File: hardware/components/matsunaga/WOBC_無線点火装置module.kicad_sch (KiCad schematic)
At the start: 24 parts, among them Q4 NPN, Q5 BS250, Q6 BS170, SW2 SW_DPDT_x2

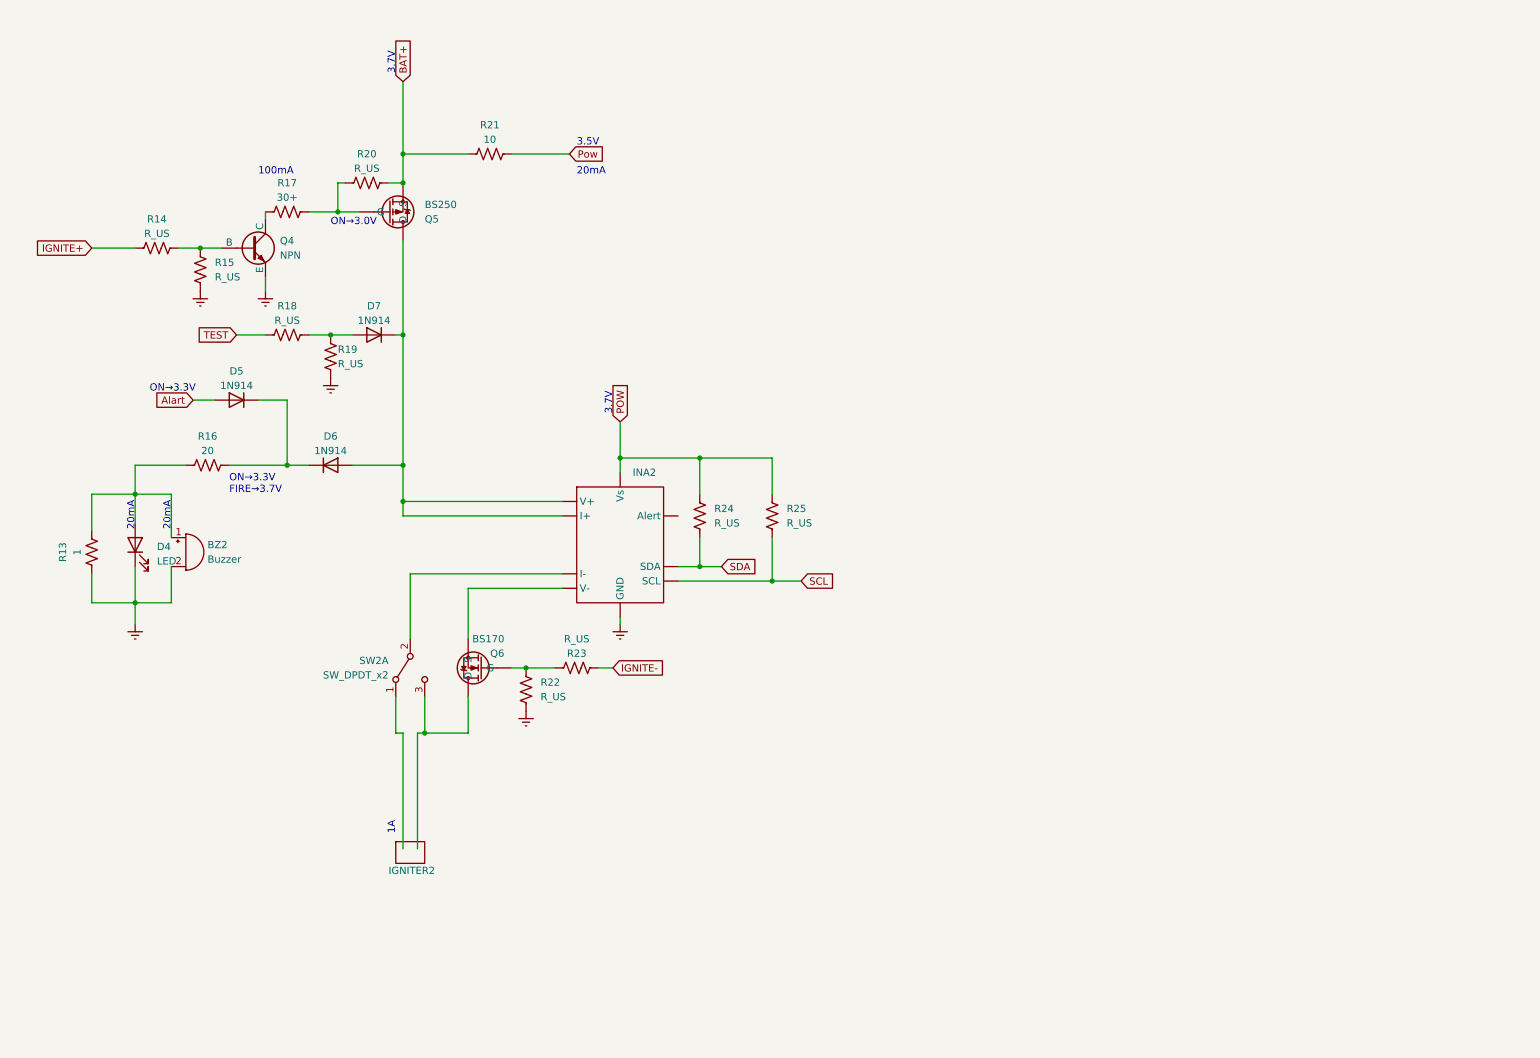
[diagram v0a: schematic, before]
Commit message: New Changes 20240111
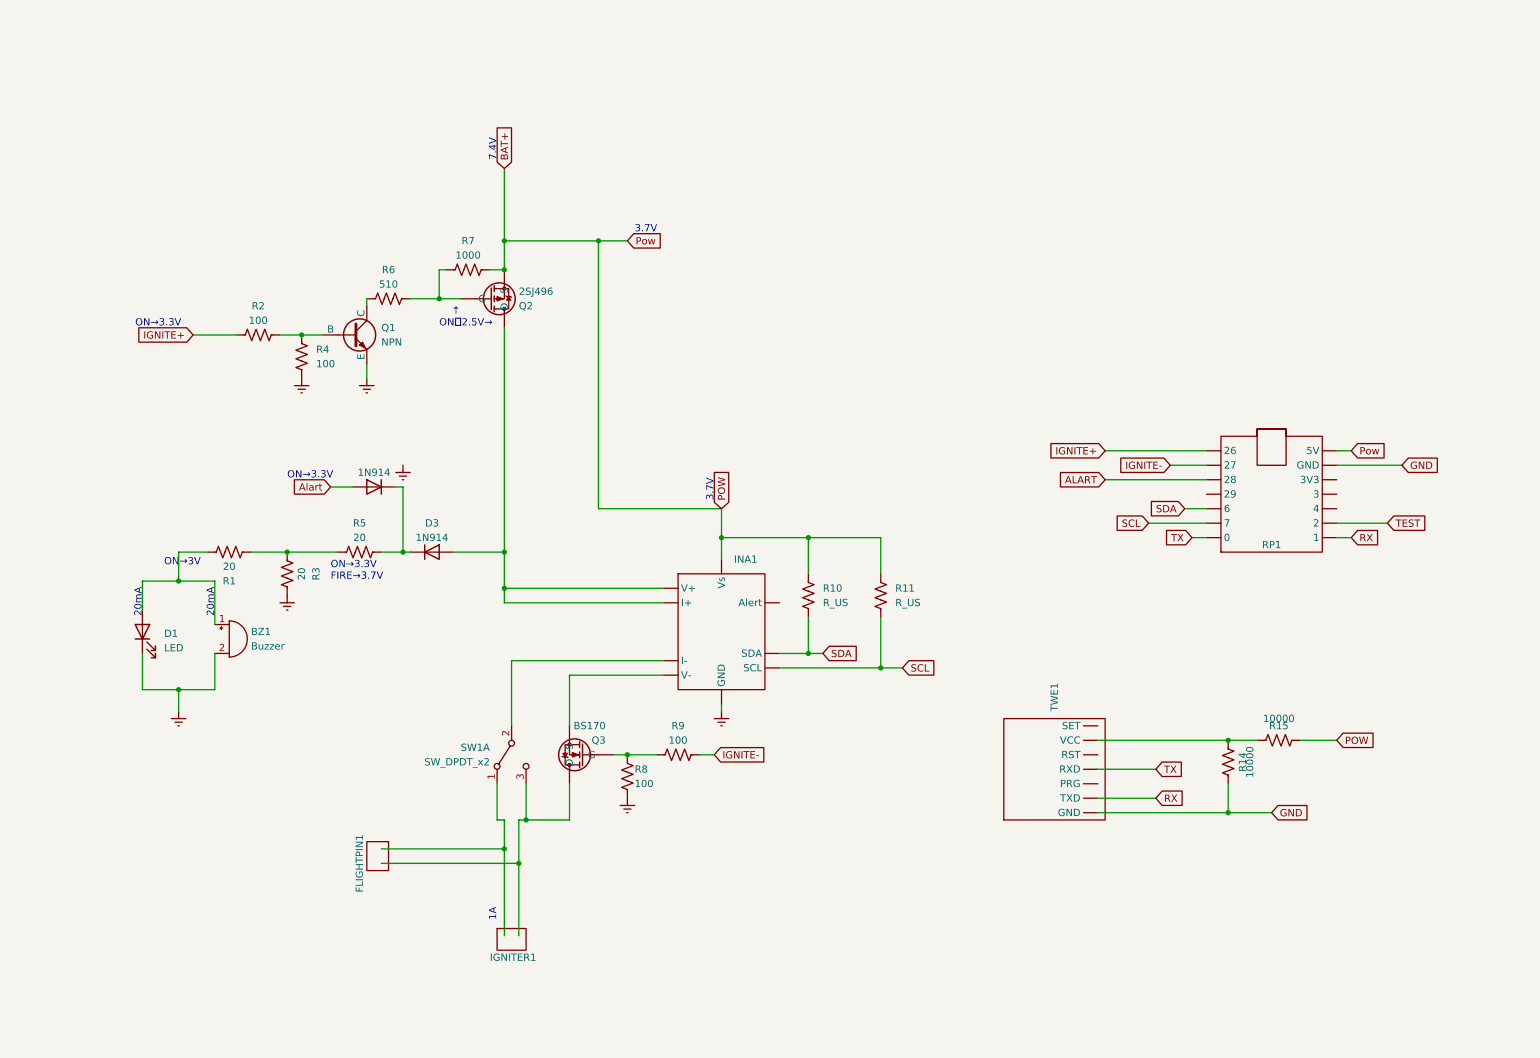
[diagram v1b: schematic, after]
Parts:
- removed BZ2: Buzzer, symbol Device:Buzzer
- removed D4: LED, symbol Device:LED
- removed D5, D6, D7: 1N914, Diode_THT:D_DO-35_SOD27_P7.62mm_Horizontal, symbol Diode:1N914
- removed IGNITER2: ~, symbol Modelrocket Igniter:SingleIgniter
- removed INA2: ~, symbol Currentmeter-Voltmeter:INA226_module
- removed Q4: NPN, symbol Simulation_SPICE:NPN
- removed Q5: BS250, Package_TO_SOT_THT:TO-92_Inline, symbol Transistor_FET:BS250
- removed Q6: BS170, Package_TO_SOT_THT:TO-92_Inline, symbol Transistor_FET:BS170
- removed R13: 1, symbol Device:R_US
- removed R16: 20, symbol Device:R_US
- removed R17: 30+, symbol Device:R_US
- removed R18, R19, R20, R22, R23, R24, R25: R_US, symbol Device:R_US
- removed R21: 10, symbol Device:R_US
- removed SW2: SW_DPDT_x2, symbol Switch:SW_DPDT_x2
- added BZ1: Buzzer, symbol Device:Buzzer
- added D1: LED, symbol Device:LED
- added D2, D3: 1N914, Diode_THT:D_DO-35_SOD27_P7.62mm_Horizontal, symbol Diode:1N914
- added FLIGHTPIN1, IGNITER1: ~, symbol Modelrocket Igniter:SingleIgniter
- added INA1: ~, symbol Currentmeter-Voltmeter:INA226_module
- added Q1: NPN, symbol Simulation_SPICE:NPN
- added Q2: 2SJ496, Package_TO_SOT_THT:TO-92_Inline, symbol Transistor_FET:BS250
- added Q3: BS170, Package_TO_SOT_THT:TO-92_Inline, symbol Transistor_FET:BS170
- added R1, R3, R5: 20, symbol Device:R_US
- added R10, R11: R_US, symbol Device:R_US
- added R2, R4, R8, R9: 100, symbol Device:R_US
- added R6: 510, symbol Device:R_US
- added R7: 1000, symbol Device:R_US
- added RP1: ~, symbol miconboard:Seeed_Xiao_RP2040
- added SW1: SW_DPDT_x2, symbol Switch:SW_DPDT_x2
- added TWE1: ~, symbol miconboard:TWELITE_UART
- R14, R15: value R_US -> 10000
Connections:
- net Alart: now also D2.2 (A)
- net BAT+: now also R15.1, INA1. (Vs), Q2.3 (S), R10.1, R11.1, R7.1, RP1. (GND)
- net Earth: now also BZ1.2 (+), D1.1 (K), INA1. (Vs), Q1.3 (E), R3.2, R4.1, R8.1; no longer R15.1
- net IGNITE+: now also R2.2, RP1. (GND); no longer R14.2
- net IGNITE-: now also R9.1, RP1. (GND)
- net SCL: now also INA1. (Vs), R11.2, RP1. (GND)
- net SDA: now also INA1. (Vs), R10.2, RP1. (GND)
- net TEST: now also RP1. (GND)
- net at R15.2: now also R14.2, TWE1. (VCC); no longer R14.1
- new net: FLIGHTPIN1., IGNITER1., SW1.1 (A)
- new net: INA1. (Vs), SW1.2 (B)
- new net: FLIGHTPIN1., IGNITER1., Q3.1 (D), SW1.3 (C)
- new net: Q3.2 (G), R8.2, R9.2
- new net: INA1. (Vs), Q3.3 (S)
- new net: D3.2 (A), INA1. (Vs), Q2.1 (D)
- new net: Q2.2 (G), R6.1, R7.2
- new net: Q1.1 (C), R6.2
- new net: BZ1.1 (-), D1.2 (A), R1.2
- new net: Q1.2 (B), R2.1, R4.2
- new net: D2.1 (K), D3.1 (K), R5.2
- new net: R1.1, R3.1, R5.1
- new net ALART: RP1. (GND)
- new net GND: R14.1, RP1. (GND), TWE1. (VCC)
- new net RX: RP1. (GND), TWE1. (VCC)
- new net TX: RP1. (GND), TWE1. (VCC)
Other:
- note added: "7.4V"
- note added: "ON→3V"
- note added: "↑ ON：2.5V→"
- note removed: "100mA"
- note removed: "3.5V"
- note removed: "ON→3.0V"

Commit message: Almost Complete
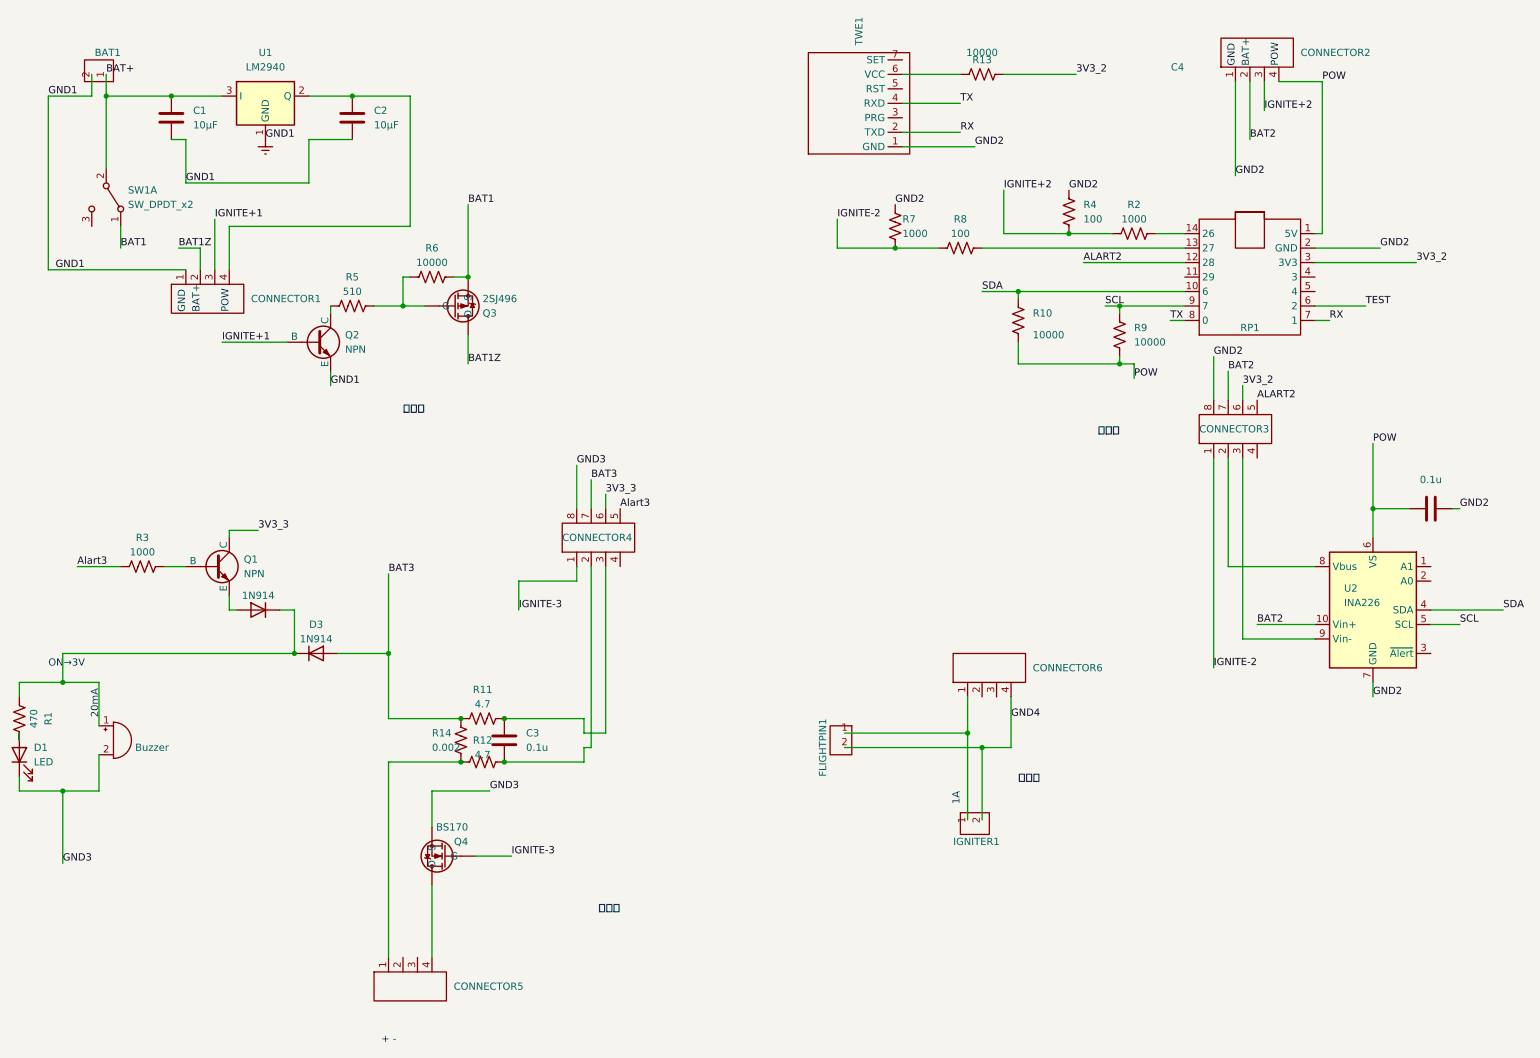
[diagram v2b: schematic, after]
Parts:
- removed INA1: ~, symbol Currentmeter-Voltmeter:INA226_module
- removed Q2: 2SJ496, Package_TO_SOT_THT:TO-92_Inline, symbol Transistor_FET:BS250
- removed Q3: BS170, Package_TO_SOT_THT:TO-92_Inline, symbol Transistor_FET:BS170
- removed R15: 10000, symbol Device:R_US
- added BAT1: ~, 2pinconnector:3pin_connector, symbol Modelrocket Igniter:SingleIgniter
- added C1, C2: 10μF, Capacitor_SMD:C_1206_3216Metric_Pad1.33x1.80mm_HandSolder, symbol Device:C
- added C3, C4: 0.1u, Capacitor_SMD:C_1206_3216Metric_Pad1.33x1.80mm_HandSolder, symbol Device:C
- added CONNECTOR1, CONNECTOR2, CONNECTOR5, CONNECTOR6: ~, MyConnector:4pin_looseconnector, symbol MyConnector:4pin_looseconnector
- added CONNECTOR3, CONNECTOR4: ~, MyConnector:8pin_looseconnector, symbol MyConnector:8pin_looseconnector
- added Q2: NPN, transistors:npn, symbol Simulation_SPICE:NPN
- added Q3: 2SJ496, Package_TO_SOT_THT:TO-92_Inline, symbol Transistor_FET:BS250
- added Q4: BS170, Package_TO_SOT_THT:TO-92_Inline, symbol Transistor_FET:BS170
- added R12: 4.7, 2pinconnector:30mil, symbol Device:R_US
- added R13: 10000, 2pinconnector:30mil, symbol Device:R_US
- added U1: LM2940, Package_TO_SOT_SMD:TO-252-3_TabPin2, symbol Regulator_Linear:IFX27001TFV50
- added U2: INA226, Package_SO:VSSOP-10_3x3mm_P0.5mm, symbol Sensor_Energy:INA226
- BZ1: footprint (none) -> Buzzer_Beeper:Buzzer_15x7.5RM7.6
- D1: footprint (none) -> LEDS:SML-D12x1
- FLIGHTPIN1, IGNITER1: footprint (none) -> 2pinconnector:2pin_connector
- Q1: footprint (none) -> transistors:npn
- R1: value 20 -> 470; footprint (none) -> 2pinconnector:30mil
- R10: value R_US -> 10000; footprint (none) -> 2pinconnector:30mil
- R11: value R_US -> 4.7; footprint (none) -> 2pinconnector:30mil
- R14: value 10000 -> 0.002; footprint (none) -> 2pinconnector:0.002
- R2: value 100 -> 1000; footprint (none) -> 2pinconnector:1.05K
- R3: value 20 -> 1000; footprint (none) -> 2pinconnector:1.05K
- R4, R8: footprint (none) -> 2pinconnector:30mil
- R5: value 20 -> 510; footprint (none) -> 2pinconnector:1.05K
- R6: value 510 -> 10000; footprint (none) -> 2pinconnector:30mil
- R7: footprint (none) -> 2pinconnector:1.05K
- R9: value 100 -> 10000; footprint (none) -> 2pinconnector:30mil
- RP1: footprint (none) -> 2pinconnector:SeeedXiaoRP2040
- SW1: footprint (none) -> 2pinconnector:SW
- TWE1: footprint (none) -> 2pinconnector:TWELITE
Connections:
- net BAT+: now also SW1.2 (B), BAT1.1, C1.1, U1.3 (I); no longer R10.1, R11.1, R7.1, RP1. (GND)
- net Earth: now also BAT1.2, C1.2, C2.2, CONNECTOR1.1, Q2.3 (E), U1.1 (GND); no longer BZ1.2 (+), D1.1 (K), Q1.3 (E), R3.2, R4.1, R8.1
- net RX: now also RP1.7 (1), TWE1.2 (TXD); no longer RP1. (GND), TWE1. (VCC)
- net SCL: now also R9.1, RP1.9 (7), U2.5 (SCL); no longer R11.2, RP1. (GND)
- net SDA: now also R10.1, RP1.10 (6), U2.4 (SDA); no longer R10.2, RP1. (GND)
- net TEST: now also RP1.6 (2); no longer RP1. (GND)
- net TX: now also RP1.8 (0), TWE1.4 (RXD); no longer RP1. (GND), TWE1. (VCC)
- net IGNITE-2: now reaches R8.2
- net IGNITE-2: now also R7.1, CONNECTOR3.1; no longer R9.2
- net BAT3: now reaches D3.2 (A)
- net BAT3: now also R11.2, R14.1, CONNECTOR4.7
- net BAT1: now reaches R6.1
- net BAT1: now also SW1.1 (A), Q3.3 (S); no longer R7.2
- net at R6.2: now also R5.1, Q3.2 (G); no longer Q1.1 (C)
- net at D1.2 (A), R1.2: no longer BZ1.1 (-)
- net at D2.1 (K), D3.1 (K): now also BZ1.1 (-), R1.1; no longer R5.2
- net at R14.2: now also CONNECTOR5.1, R12.2; no longer TWE1. (VCC)
- removed net ALART: RP1. (GND)
- net Alart: no longer names the net of D2.2 (A)
- net Alart: now also Q1.3 (E)
- removed net GND: R14.1, RP1. (GND), TWE1. (VCC)
- net IGNITE+ renamed IGNITE+2
- net IGNITE+2: now also R4.1, CONNECTOR2.3; no longer RP1. (GND)
- removed net IGNITE-: R9.1, RP1. (GND)
- new net: Q2.1 (C), R5.2
- new net: CONNECTOR5.4, Q4.1 (D)
- new net: R8.1, RP1.13 (27)
- new net: R2.1, RP1.14 (26)
- new net: CONNECTOR6.1, FLIGHTPIN1.1, IGNITER1.1
- new net: CONNECTOR3.2, U2.8 (Vbus)
- new net: CONNECTOR3.3, U2.9 (Vin-)
- new net: Q1.2 (B), R3.1
- new net: R13.2, TWE1.6 (VCC)
- new net: C2.1, CONNECTOR1.4, U1.2 (Q)
- new net: C3.2, CONNECTOR4.2, R12.1
- new net: C3.1, CONNECTOR4.3, R11.1
- new net 3V3_2: CONNECTOR3.6, R13.1, RP1.3 (3V3)
- new net 3V3_3: CONNECTOR4.6, Q1.1 (C)
- new net ALART2: CONNECTOR3.5, RP1.12 (28)
- new net Alart3: CONNECTOR4.5, R3.2
- new net BAT1Z: CONNECTOR1.2, Q3.1 (D)
- new net BAT2: CONNECTOR2.2, CONNECTOR3.7, U2.10 (Vin+)
- new net GND2: C4.2, CONNECTOR2.1, CONNECTOR3.8, R4.2, R7.2, RP1.2 (GND), TWE1.1 (GND), U2.7 (GND)
- new net GND3: BZ1.2 (+), CONNECTOR4.8, D1.1 (K), Q4.3 (S)
- new net GND4: CONNECTOR6.4, FLIGHTPIN1.2, IGNITER1.2
- new net IGNITE+1: CONNECTOR1.3, Q2.2 (B)
- new net IGNITE-3: CONNECTOR4.1, Q4.2 (G)
- new net POW: C4.1, CONNECTOR2.4, R10.2, R9.2, RP1.1 (5V), U2.6 (VS)
- now unconnected: SW1.3 (C)
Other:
- note added: "+ -"
- note added: "BAT+"
- note added: "GND"
- note added: "POW"
- note added: "１枚目"
- note added: "２枚目"
- note added: "３枚目"
- note added: "４枚目"
- note removed: "3.7V"
- note removed: "7.4V"
- note removed: "ON→3.3V"
- note removed: "ON→3.3V FIRE→3.7V"
- note removed: "↑ ON：2.5V→"
